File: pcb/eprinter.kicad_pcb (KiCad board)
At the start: 4 copper layers, 28 x 70 mm, 55 parts, among them J1 USB_C_Receptacle_USB2.0_16P, J2 AFC07-S24FCC-00, J3 Conn_01x02_Pin, Q1 Si2301, Q2 BSS138, SW1 SW_PUSH, SW2 SW_PUSH, U1 ESP32-C3-WROOM-02, U2 LM3480-5.0, U3 LM66100DCK, U4 MIC841HYC5, U5 XC6220B331MR

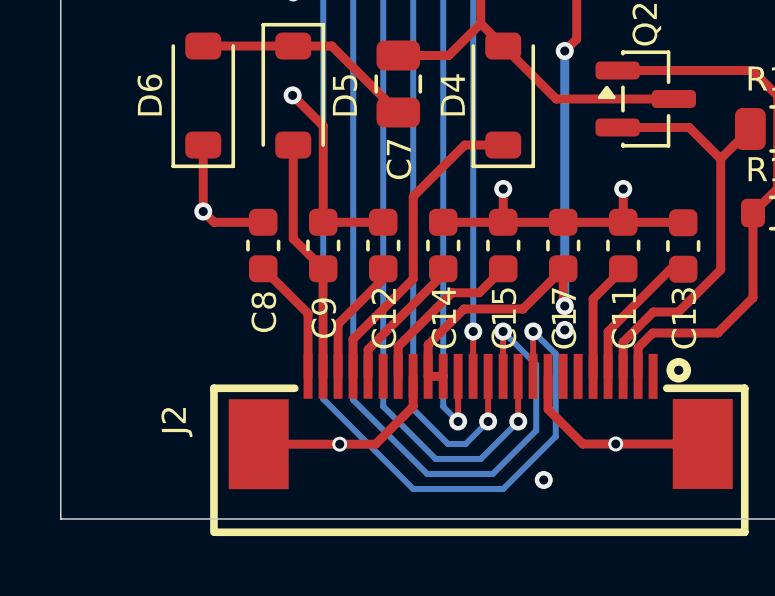
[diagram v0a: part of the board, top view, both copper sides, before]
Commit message: Finish PCB v1
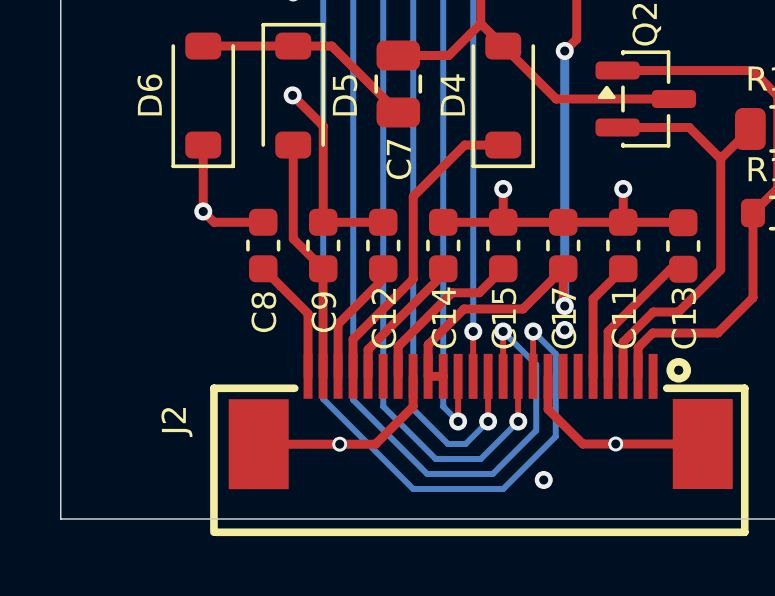
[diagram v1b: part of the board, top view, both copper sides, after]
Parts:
- R16: value 3M -> 2M
- R17: value 430k -> 330k
- R18: value 1.5M -> 1M
